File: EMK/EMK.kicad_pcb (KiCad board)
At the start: 4 copper layers, 114.1 x 92.5 mm, 122 parts, among them J1 USB_C_Receptacle_USB2.0_14P, J2 Conn_01x02_Socket, J3 Conn_ARM_JTAG_SWD_10, Q1 Si2371EDS, Q2 Si2371EDS, SW1 SW_Nidec_CAS-120A1, SW10 MX3, SW11 MX7, SW12 MX11, SW13 MX15, SW14 MX4, SW15 MX8, SW16 MX12, SW17 MX16, SW18 SW_Push, SW19 SW_Nidec_CAS-120A1, SW2 MX1, SW20 Mode Switch, SW3 MX5, SW4 MX9, SW5 MX13, SW6 MX2, SW7 MX6, SW8 MX10, SW9 MX14, U1 nRF52840-QFAA, U2 15nH, U3 TPS62822DLC, U4 USBLC6-2SC6, U5 TP4057, Y1 Crystal_32.768kHz, Y2 Crystal_32mHz

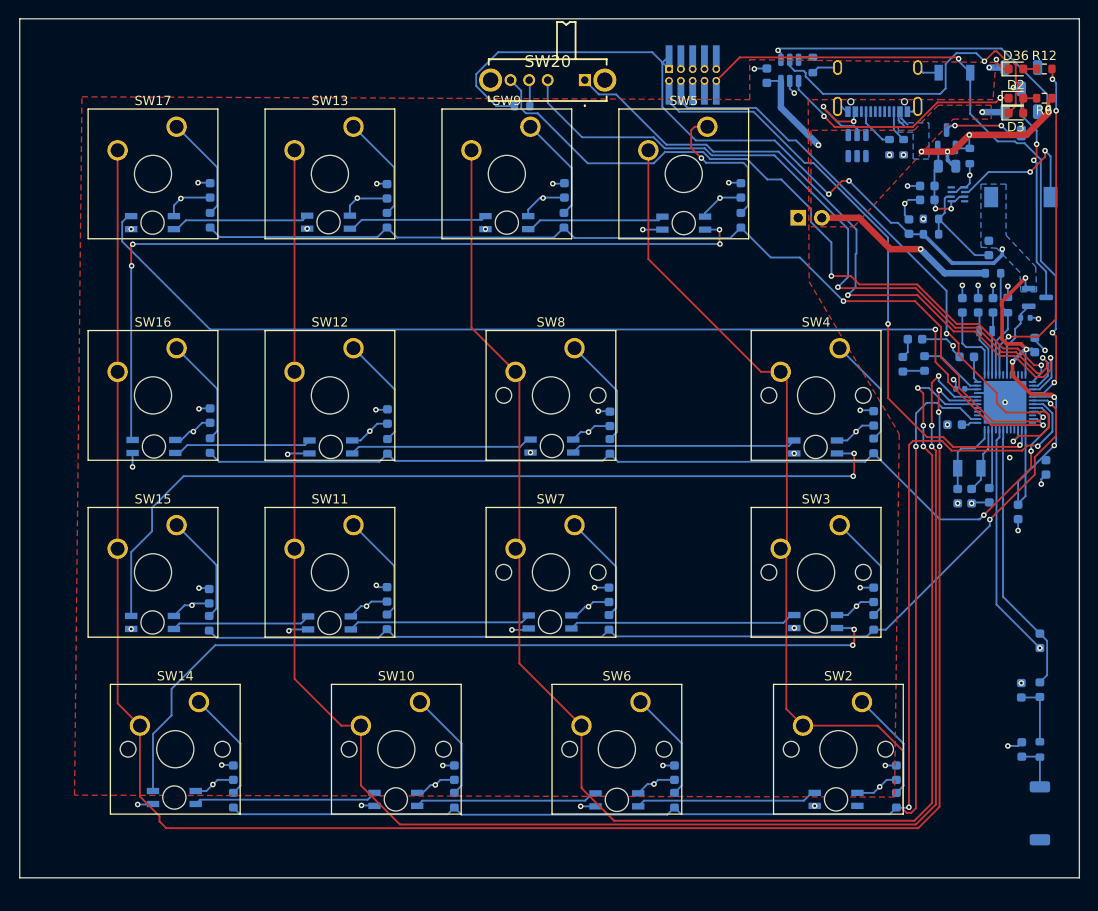
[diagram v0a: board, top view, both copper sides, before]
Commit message: Finalização
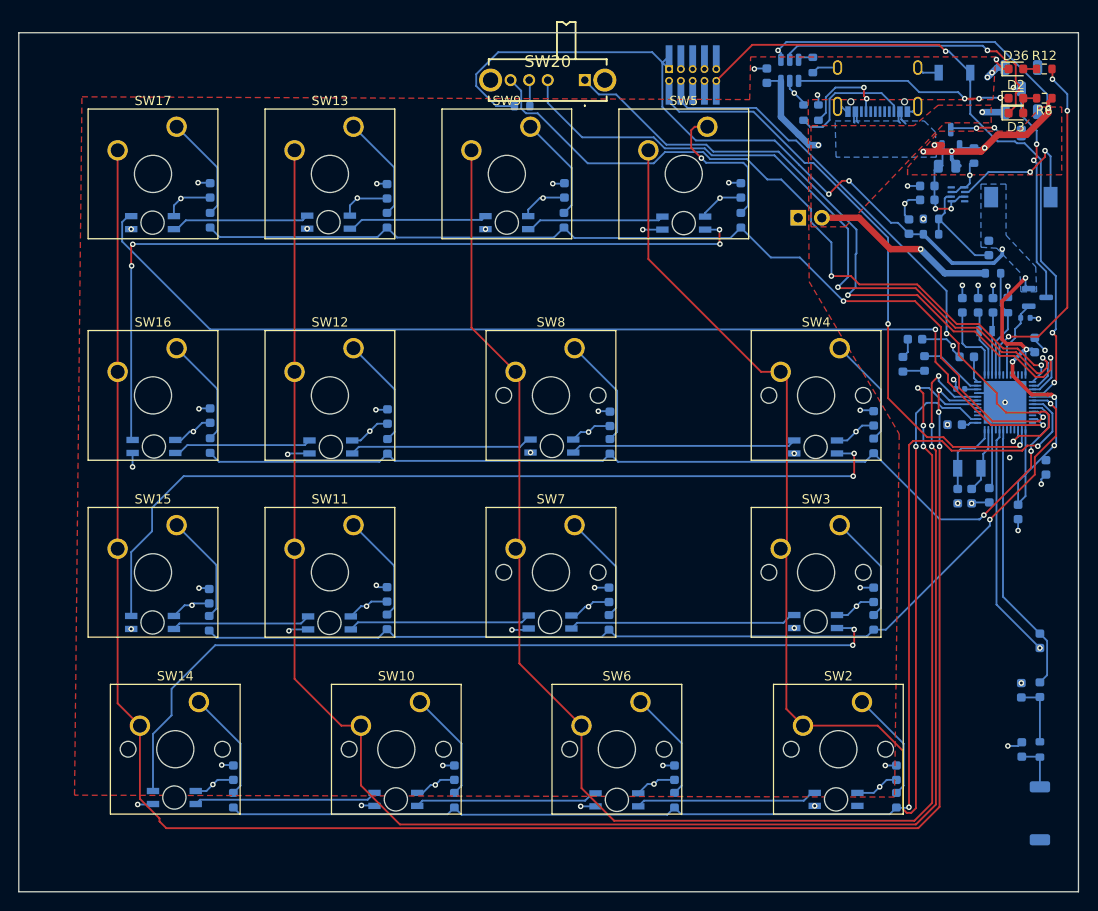
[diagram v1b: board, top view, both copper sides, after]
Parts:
- removed U4: USBLC6-2SC6, Package_TO_SOT_SMD:SOT-23-6
- moved R2 11.4 mm to (121.9, 32.5), turned to 90 degrees
- moved R1 8.51 mm to (123.5, 32.5), turned to 90 degrees
- moved Q1 0.45 mm to (137.8, 35.3)
- moved R3 0.45 mm to (140.2, 37.1)
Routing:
- net Net-(J1-CC2): track 3.44 -> 14.1 mm
- net VBUS: track 71.0 -> 63.2 mm, vias 7 -> 6
- net Net-(J1-CC1): track 4.49 -> 10.1 mm, vias 0 -> 2
- net Net-(D3-K): track 37.1 -> 32.0 mm
- net Net-(D2-K): track 26.6 -> 23.5 mm, vias 3 -> 4
- net GND: track 106.6 -> 109.4 mm, vias 59 -> 58
- net ON_LED: track 37.8 -> 38.8 mm
- net NRST: track 72.2 -> 73.1 mm
- net Net-(Q1-D): track 8.58 -> 7.92 mm
- net RGB_VDD: track 78.9 -> 79.6 mm, vias 17 -> 18
- net VBAT: track 32.8 -> 33.4 mm
- net Net-(D1-K): track 11.0 -> 11.6 mm
- added copper zone on F.Cu, net VBUS
